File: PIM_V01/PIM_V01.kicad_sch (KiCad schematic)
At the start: 98 parts, among them J1 Conn_01x06, J10 Conn_02x08_Odd_Even, J4 USB_C_Receptacle_USB2.0_14P, J5 Conn_01x04, J6 Conn_01x04, J7 Conn_02x03_Odd_Even, J8 Conn_01x02, J9 Conn_02x08_Odd_Even, Q1 SQJ407EP-T1_GE3, Q2 PMOS, Q3 PMOS, Q4 NMOS, SW1 SW_Push, U1 TPS259541DSGR, U11 AP2112K-3.3, U13 MT29F1G01ABAFDWB-IT_F, U14 MB85RS256B, U2 USBLC6-2SC6, U3 STM32H7A3VITx, Y1 Crystal_GND24_Small

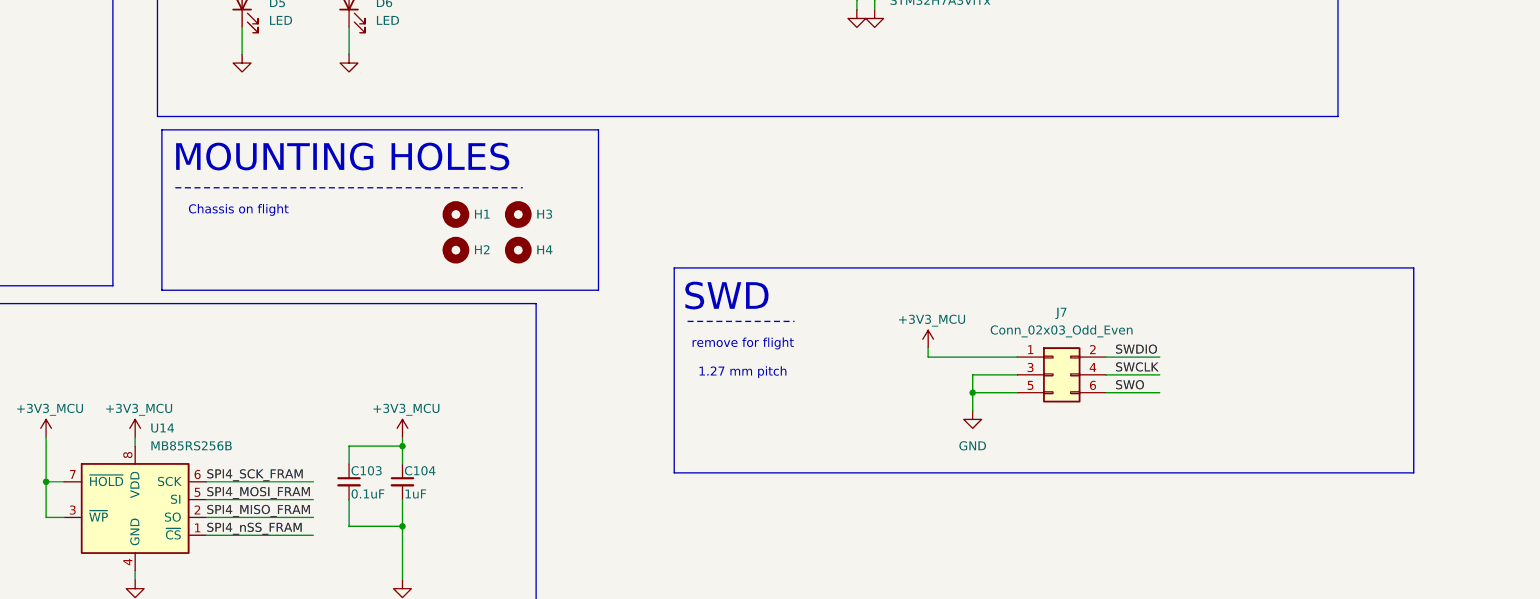
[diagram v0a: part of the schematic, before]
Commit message: V01 RELEASE. Gerbers created to order RAW PCB
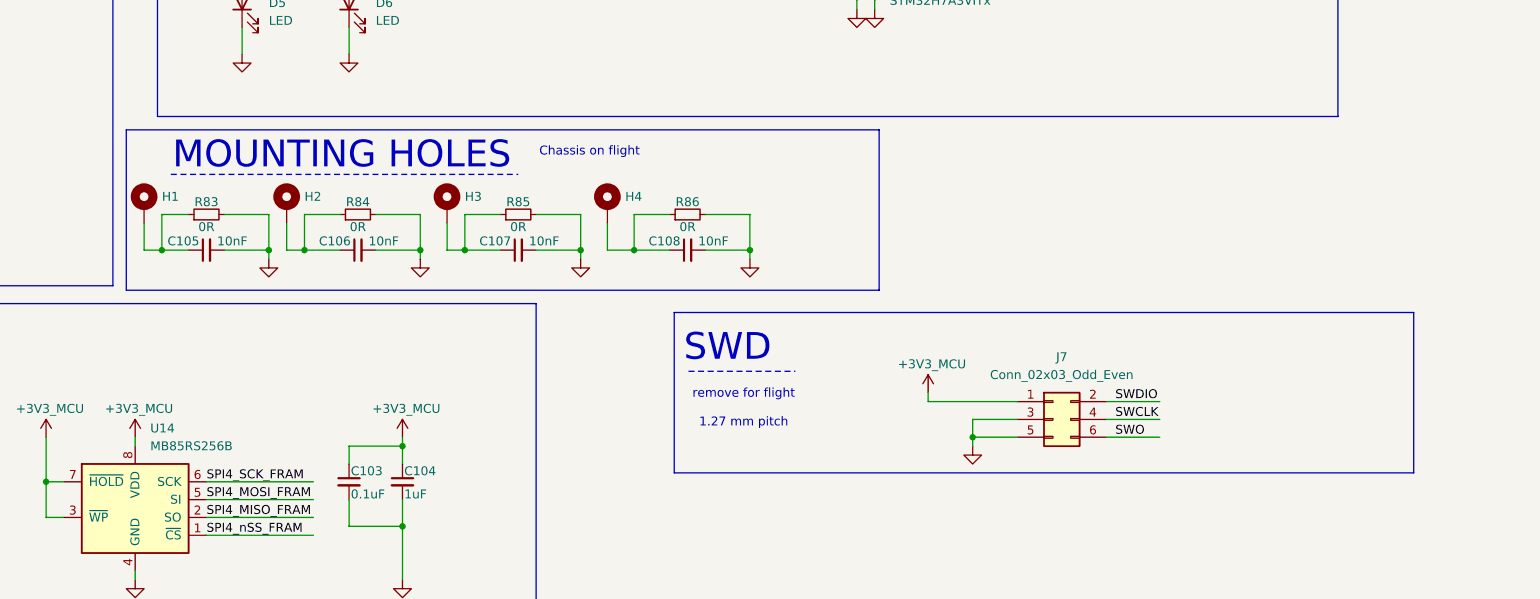
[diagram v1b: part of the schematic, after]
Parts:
- removed H1, H2, H3, H4: MountingHole, MountingHole:MountingHole_2.2mm_M2, symbol Mechanical:MountingHole
- added C105, C106, C107, C108: 10nF, Capacitor_SMD:C_0603_1608Metric, symbol Device:C_Small
- added H1, H2, H3, H4: MountingHole_Pad, MountingHole:MountingHole_2.2mm_M2_Pad, symbol Mechanical:MountingHole_Pad
- added R83, R84, R85, R86: 0R, Resistor_SMD:R_0603_1608Metric, symbol Device:R_Small
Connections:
- net GND: now also C105.2, C106.2, C107.2, C108.2, R83.2, R84.2, R85.2, R86.2
- new net: C107.1, H3.1, R85.1
- new net: C106.1, H2.1, R84.1
- new net: C105.1, H1.1, R83.1
- new net: C108.1, H4.1, R86.1
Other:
- moved on the sheet: J7
